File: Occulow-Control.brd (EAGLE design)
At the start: 38.1 x 101.6 mm, 40 parts, among them J1 CORTEX_DEBUG_PTH, T1 DMP3010LK3, T2 DMP3010LK3, T3 DMP3010LK3

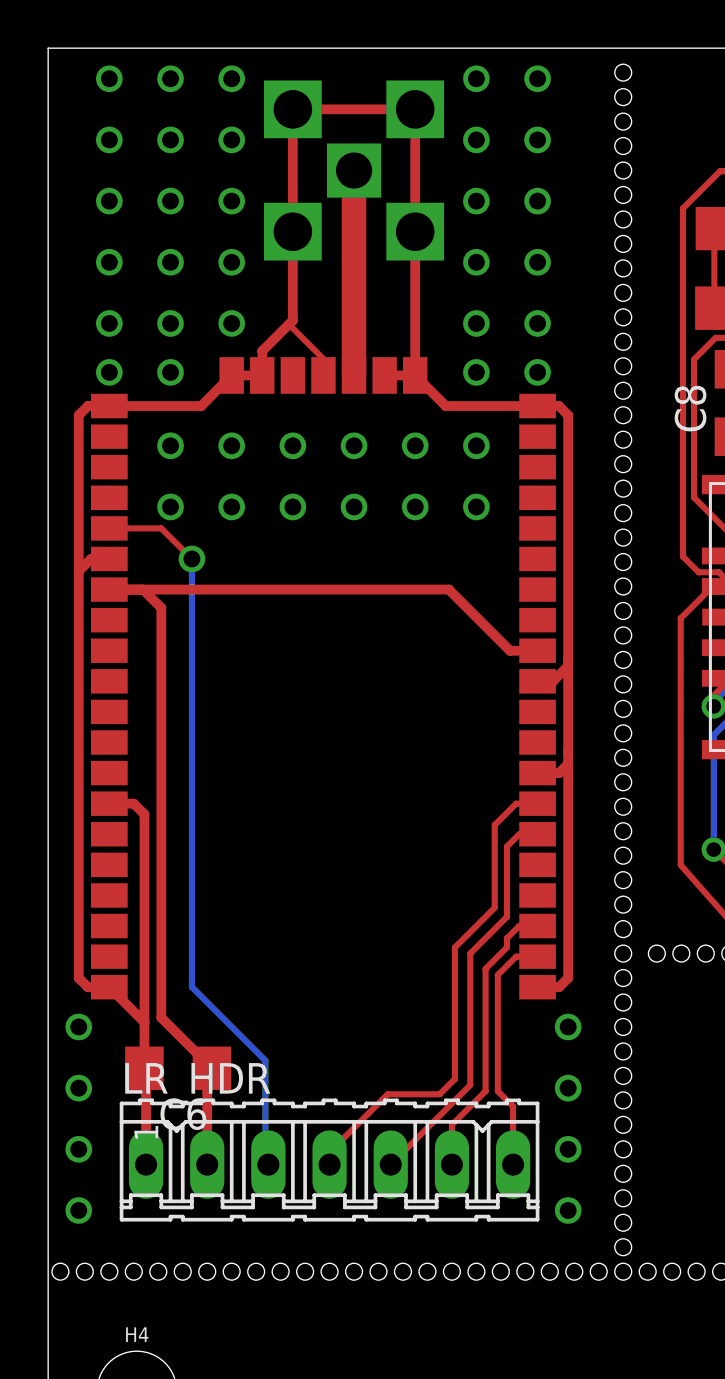
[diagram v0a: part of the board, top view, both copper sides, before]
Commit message: Ground plane
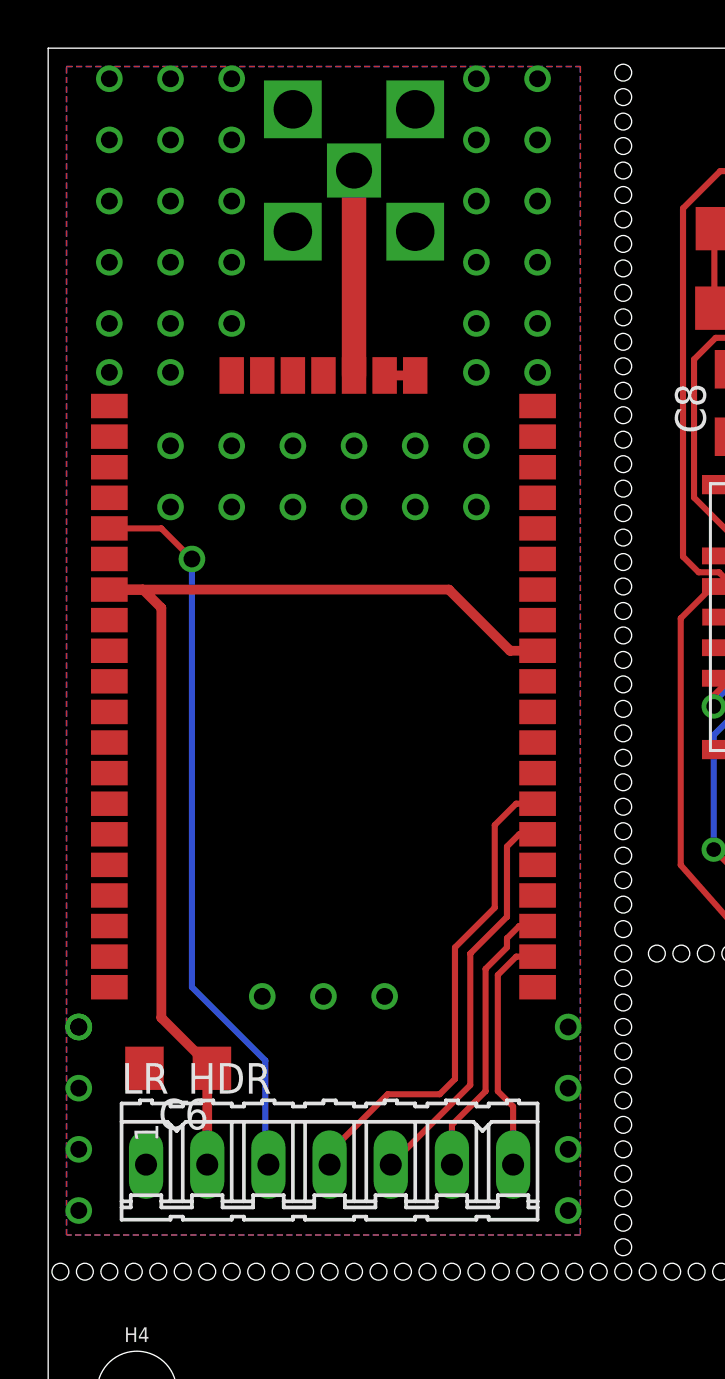
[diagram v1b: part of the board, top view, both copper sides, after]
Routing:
- net LR_GND: track 119.3 -> 1.36 mm, vias 0 -> 53
- added copper zone on layer 1, net LR_GND
- added copper zone on layer 16, net LR_GND
